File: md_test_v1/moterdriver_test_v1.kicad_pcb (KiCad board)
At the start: 2 copper layers, 47 x 37.5 mm, 20 parts, among them J1 Conn_01x02_Socket, J2 Conn_01x03_Socket, J3 Conn_01x02_Socket, Q1 rs6, Q2 rs6, Q3 rs6, Q4 rs6, U1 DRV8701PRGER

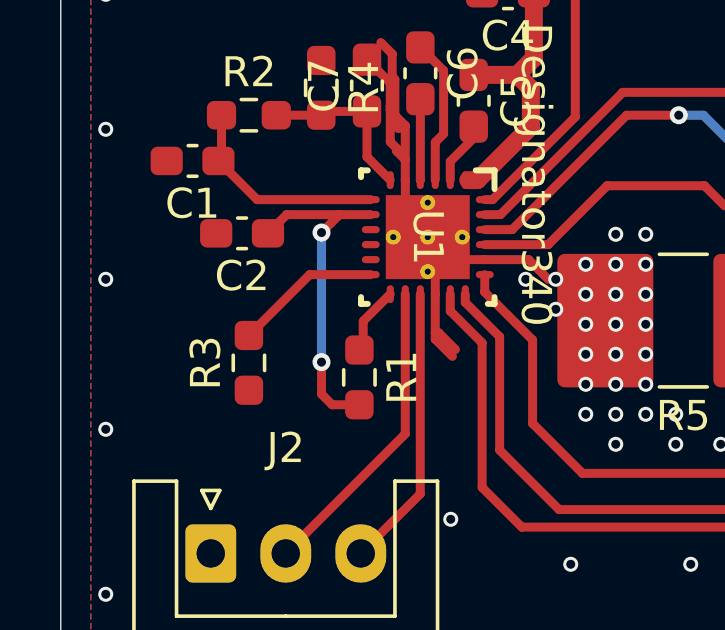
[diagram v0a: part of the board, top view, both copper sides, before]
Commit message: md改良(ちょっと前にしたやつ上げ忘れ)
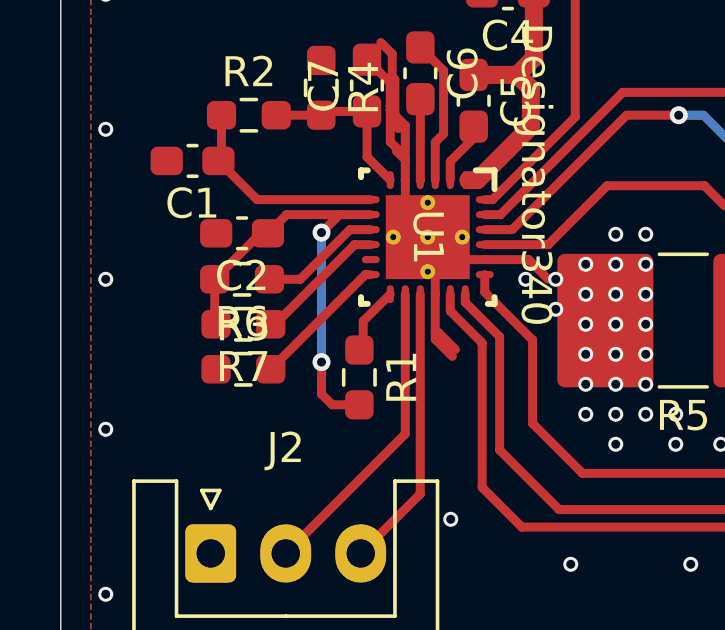
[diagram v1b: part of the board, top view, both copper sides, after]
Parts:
- added R6: 10k, Resistor_SMD:R_0603_1608Metric_Pad0.98x0.95mm_HandSolder, F.Cu at (56.0, 71.0)
- added R7: 10k, Resistor_SMD:R_0603_1608Metric_Pad0.98x0.95mm_HandSolder, F.Cu at (56.1, 72.5)
- C1, C2: value 0.1uf -> 1uF
- moved R3 0.28 mm to (56.1, 74.0), turned to 0 degrees
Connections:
- U1 pad V: (no net) -> GND1
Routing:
- net /sns_out: track 0.00 -> 4.43 mm
- net /faultN_out: track 0.00 -> 4.06 mm
- net Net-(U1-DVDD): track 11.3 -> 15.2 mm

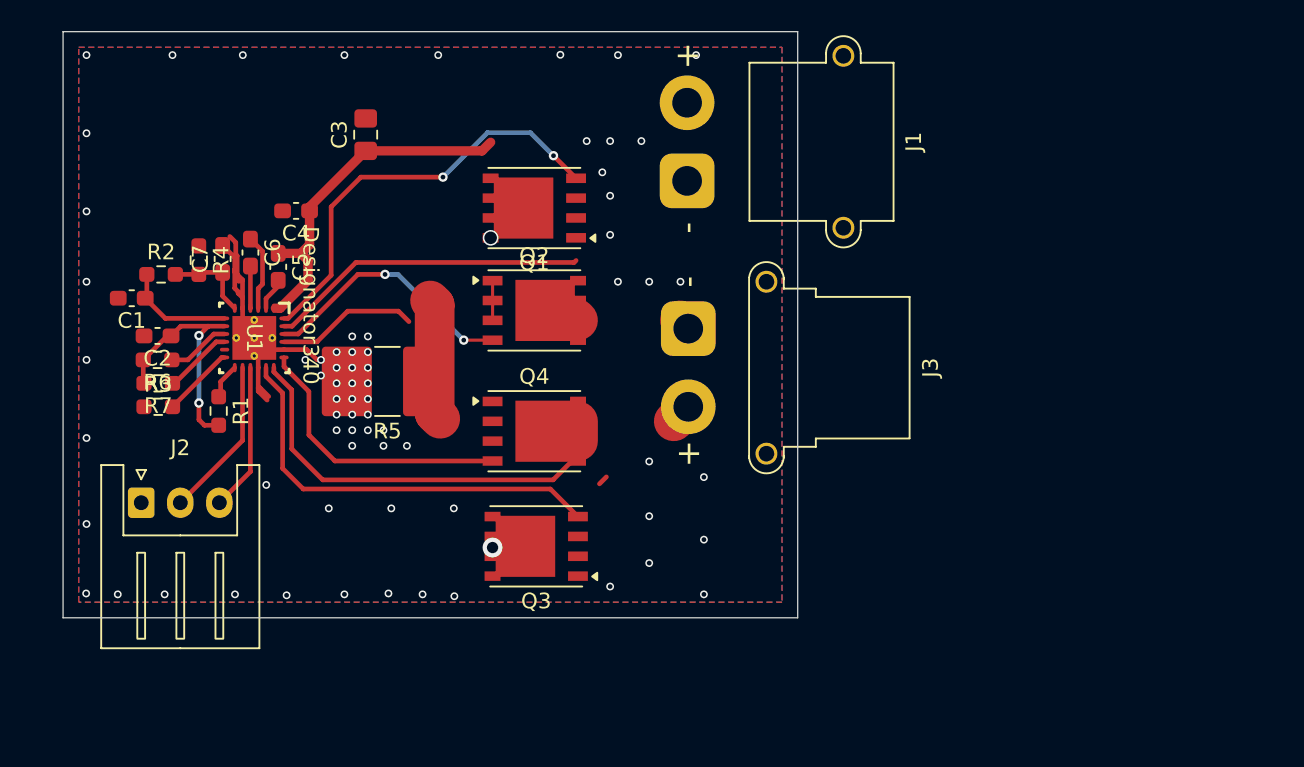
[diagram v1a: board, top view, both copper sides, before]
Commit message: MDを設計した(できたと思っている)
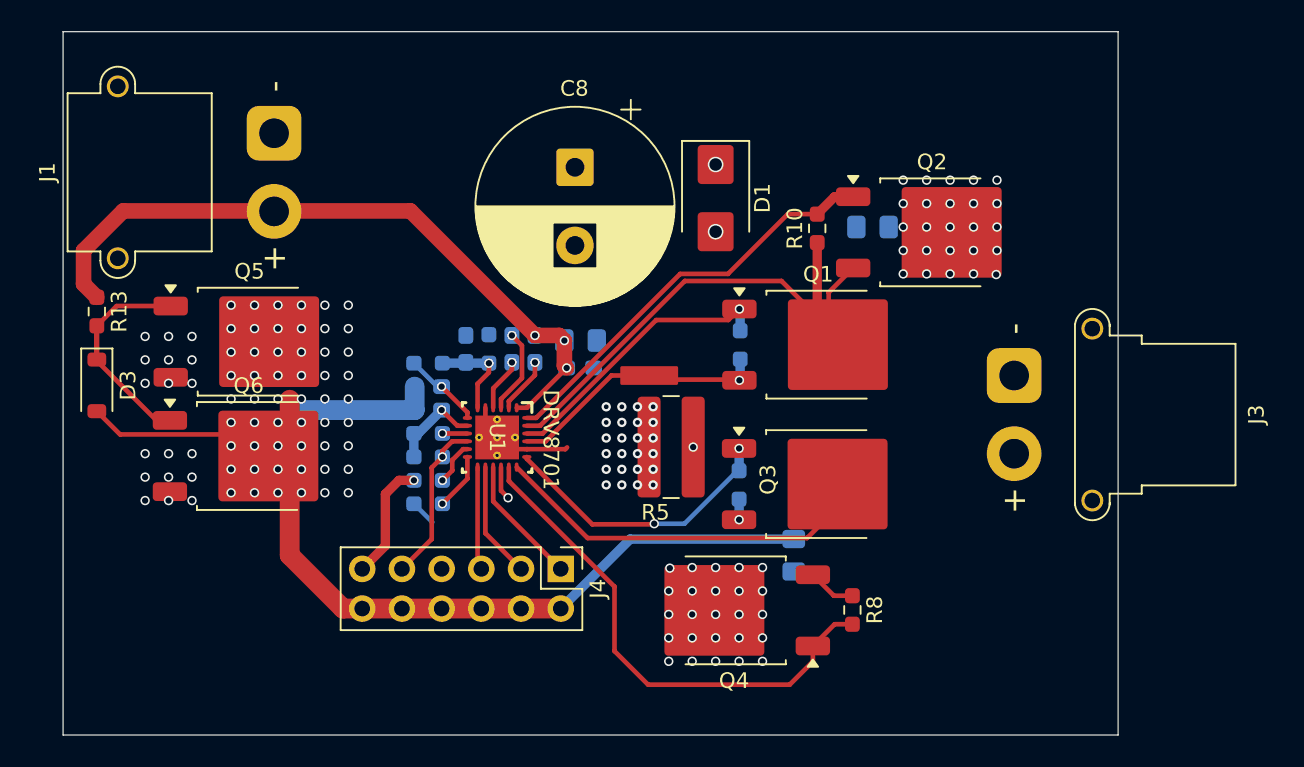
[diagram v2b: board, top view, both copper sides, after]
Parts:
- removed J2: Conn_01x03_Socket, Connector_JST:JST_XH_S3B-XH-A_1x03_P2.50mm_Horizontal
- removed R1: 10k, Resistor_SMD:R_0603_1608Metric_Pad0.98x0.95mm_HandSolder
- added C10: 10uF, Capacitor_SMD:C_0805_2012Metric_Pad1.18x1.45mm_HandSolder, B.Cu at (101.8, 62.5)
- added C8: 250uF, Capacitor_THT:CP_Radial_D12.5mm_P5.00mm, F.Cu at (82.8, 58.7)
- added C9: 10uF, Capacitor_SMD:C_0805_2012Metric_Pad1.18x1.45mm_HandSolder, B.Cu at (96.8, 83.5)
- added D1: D_TVS, Diode_SMD:D_SMB, F.Cu at (91.8, 60.6)
- added D3: D_Zener, Diode_SMD:D_SOD-123, F.Cu at (52.2, 72.6)
- added J4: Conn_02x06_Odd_Even, Connector_PinHeader_2.54mm:PinHeader_2x06_P2.54mm_Vertical, F.Cu at (81.8, 84.4)
- added Q5: Q_NMOS_GDS, Package_TO_SOT_SMD:TO-252-2, F.Cu at (61.9, 69.8)
- added Q6: Q_NMOS_GDS, Package_TO_SOT_SMD:TO-252-2, F.Cu at (61.9, 77.2)
- added R10: 10k, Resistor_SMD:R_0603_1608Metric_Pad0.98x0.95mm_HandSolder, F.Cu at (98.2, 62.6)
- added R11: 10k, Resistor_SMD:R_0603_1608Metric_Pad0.98x0.95mm_HandSolder, B.Cu at (93.3, 70.0)
- added R12: 1k, Resistor_SMD:R_0603_1608Metric_Pad0.98x0.95mm_HandSolder, B.Cu at (73.4, 78.7)
- added R13: 10k, Resistor_SMD:R_0603_1608Metric_Pad0.98x0.95mm_HandSolder, F.Cu at (52.2, 67.9)
- added R8: 10k, Resistor_SMD:R_0603_1608Metric_Pad0.98x0.95mm_HandSolder, F.Cu at (100.5, 87.0)
- added R9: 10k, Resistor_SMD:R_0603_1608Metric_Pad0.98x0.95mm_HandSolder, B.Cu at (93.2, 79.0)
- C1, C2, C3, C4, C5, C6, C7, R4, R6, R7: moved to B.Cu
- Q1, Q2, Q3, Q4: value rs6 -> Q_NMOS_GDS; footprint Package_SO:PowerPAK_SO-8_Single -> Package_TO_SOT_SMD:TO-252-2
- R2: value 70k -> 18k; moved to B.Cu
- R3: value 75k -> 200k; moved to B.Cu
- R5: value 10mi -> 2m; footprint Resistor_SMD:R_2816_7142Metric_Pad3.20x4.45mm_HandSolder -> Resistor_SMD:R_1225_3264Metric_Pad1.47x6.45mm_HandSolder
- U1: footprint drv8701prger:RGE0024F -> drv8701:RGE0024F
- moved J1 26.6 mm to (63.5, 56.5), turned to 90 degrees
- moved Q2 25.9 mm to (105.6, 62.8)
- moved J3 21.1 mm to (110.8, 72.0)
- moved C4 20.8 mm to (83.1, 71.5), turned to 0 degrees
- moved Q1 20.2 mm to (98.3, 70.0), turned to 0 degrees
- moved C1 19.8 mm to (73.4, 72.7)
- moved R4 19.4 mm to (77.2, 70.3)
- moved C3 19.0 mm to (83.1, 69.8), turned to 0 degrees
- moved R5 18.6 mm to (88.9, 76.6)
- moved Q3 18.5 mm to (98.3, 78.9), turned to 0 degrees
- moved R3 18.4 mm to (73.4, 80.2)
- moved R2 18.0 mm to (73.4, 71.2)
- moved C2 18.0 mm to (73.4, 74.2)
- moved R6 17.9 mm to (73.4, 75.7)
- moved R7 17.9 mm to (73.4, 77.2)
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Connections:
- J1 pad 1: GND1 -> GND
- Q1 pad 1: Net-(J3-Pin_1) -> Net-(Q1-G)
- Q1 pad 3: Net-(J3-Pin_1) -> Net-(Q1-S)
- Q2 pad 1: Net-(U1-SP) -> Net-(Q2-G)
- Q2 pad 2: Net-(U1-SP) -> +24V
- Q2 pad 3: Net-(U1-SP) -> Net-(J3-Pin_1)
- Q3 pad 1: Net-(J3-Pin_2) -> Net-(Q3-G)
- Q3 pad 3: Net-(J3-Pin_2) -> Net-(Q1-S)
- Q4 pad 1: Net-(U1-SP) -> Net-(Q4-G)
- Q4 pad 2: Net-(U1-SP) -> +24V
- Q4 pad 3: Net-(U1-SP) -> Net-(J3-Pin_2)
- R5 pad 1: Net-(U1-SP) -> Net-(Q1-S)
- U1 pad 17: Net-(Q3-G) -> Net-(Q4-G)
- U1 pad 19: Net-(Q4-G) -> Net-(Q3-G)
- U1 pad 21: Net-(U1-SP) -> Net-(Q1-S)
- U1 pad 22: Net-(Q2-G) -> Net-(Q1-G)
- U1 pad 24: Net-(Q1-G) -> Net-(Q2-G)
- U1 pad V: GND1 -> (no net)
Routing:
- net GND1: track 20.7 -> 78.8 mm, vias 70 -> 80
- net Net-(U1-SP): track 36.2 -> 0.00 mm
- net +24V: track 69.0 -> 44.7 mm, vias 2 -> 54
- net Net-(J3-Pin_2): track 44.0 -> 26.9 mm
- net Net-(Q1-S): track 0.00 -> 16.0 mm, vias 0 -> 3
- net Net-(D3-K): track 0.00 -> 15.9 mm
- net Net-(Q4-G): track 18.1 -> 32.9 mm
- net Net-(Q2-G): track 16.4 -> 26.7 mm, vias 2 -> 0
- net Net-(U1-DVDD): track 15.2 -> 5.96 mm, vias 2 -> 1
- net Net-(Q1-G): track 27.4 -> 18.3 mm, vias 2 -> 1
- net Net-(Q3-G): track 27.1 -> 18.3 mm, vias 0 -> 2
- net Net-(J4-Pin_11): track 0.00 -> 7.59 mm, vias 0 -> 1
- net /sns_out: track 4.43 -> 10.5 mm, vias 0 -> 1
- net /sleepN_in: track 2.16 -> 6.61 mm
- net /pwm_in2: track 10.3 -> 7.45 mm
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- removed copper zone on B.Cu, net GND1
- removed copper zone on F.Cu, net GND1
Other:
- board size 47 x 37.5 mm -> 67.5 x 45 mm
